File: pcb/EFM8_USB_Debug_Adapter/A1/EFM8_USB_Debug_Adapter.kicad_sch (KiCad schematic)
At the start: 27 parts, among them J100 EFM8 IDC Debug Header, J110 2137160001, J111 TTL-232R Header, J120 31230102, J130 EFM8 USB 8-Bit Debug Header, J131 Conn_01x02_Male, Q110 SI3443CDV-T1-GE3, Q111 DMMT5401, Q120 SI3443CDV-T1-GE3, Q121 DMMT5401, Q130 SI3443CDV-T1-GE3, Q131 DMMT5401

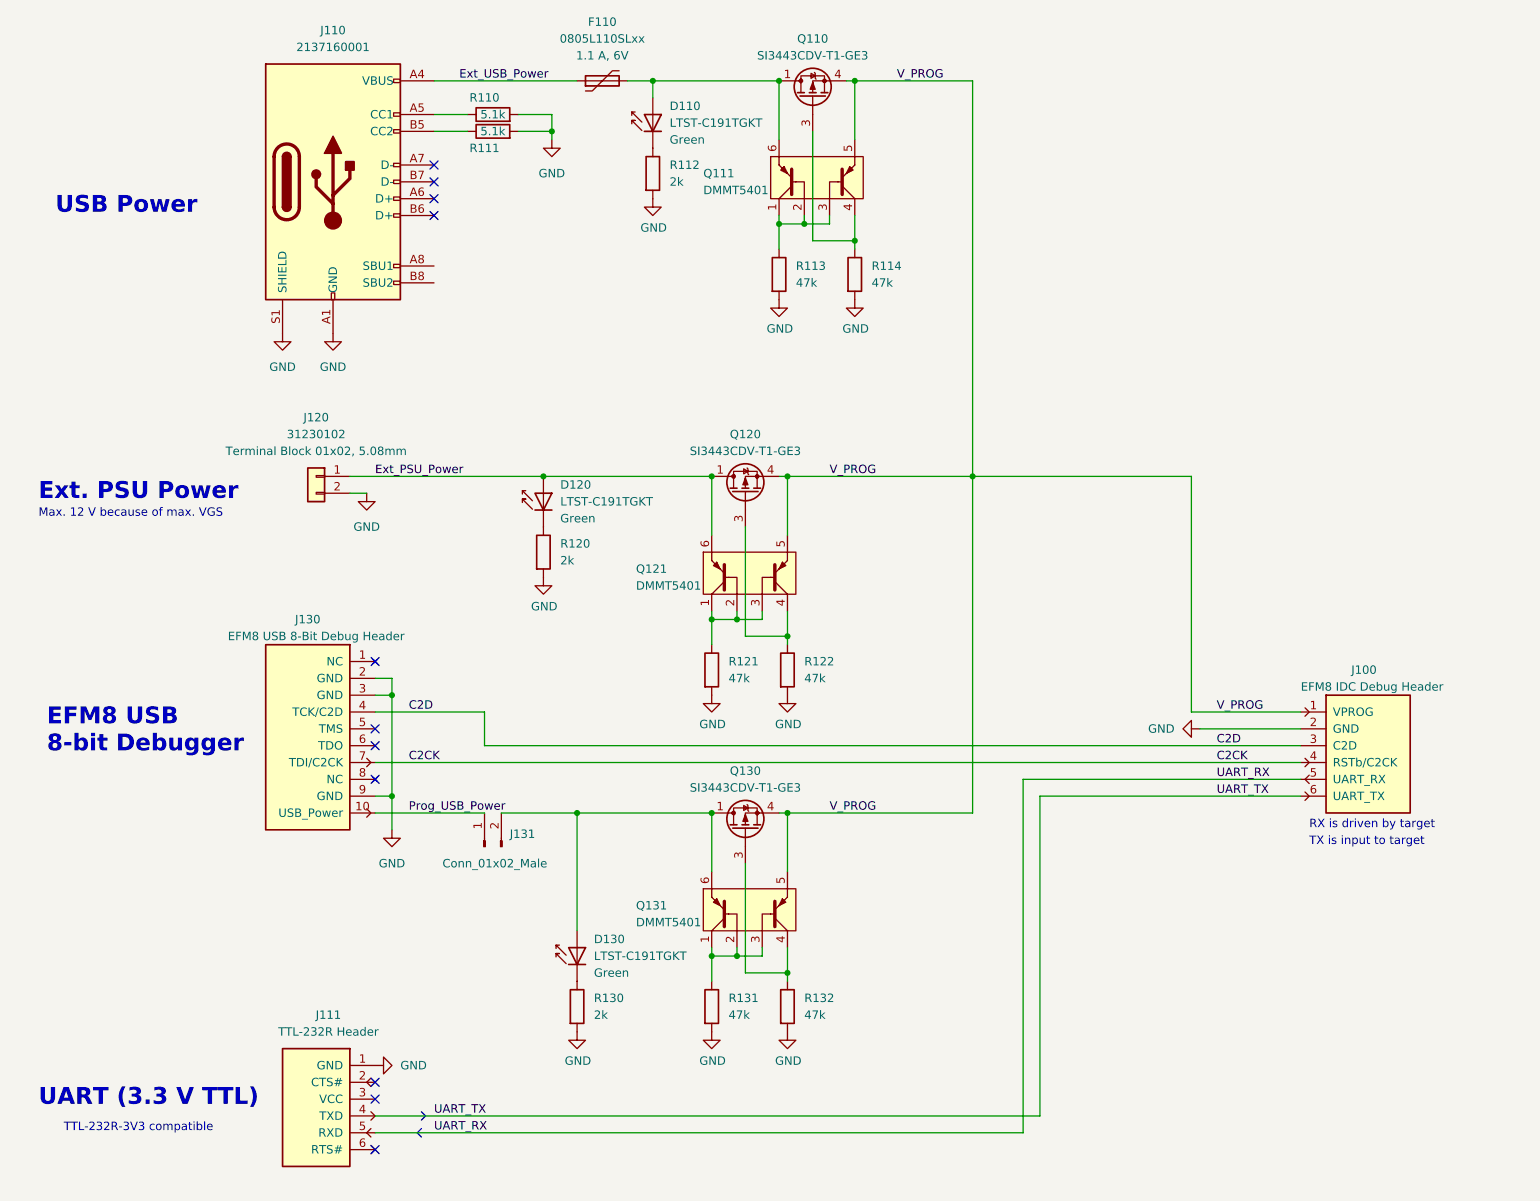
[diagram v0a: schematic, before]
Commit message: PCB bearbeitet, FreeCAD Projet angelegt
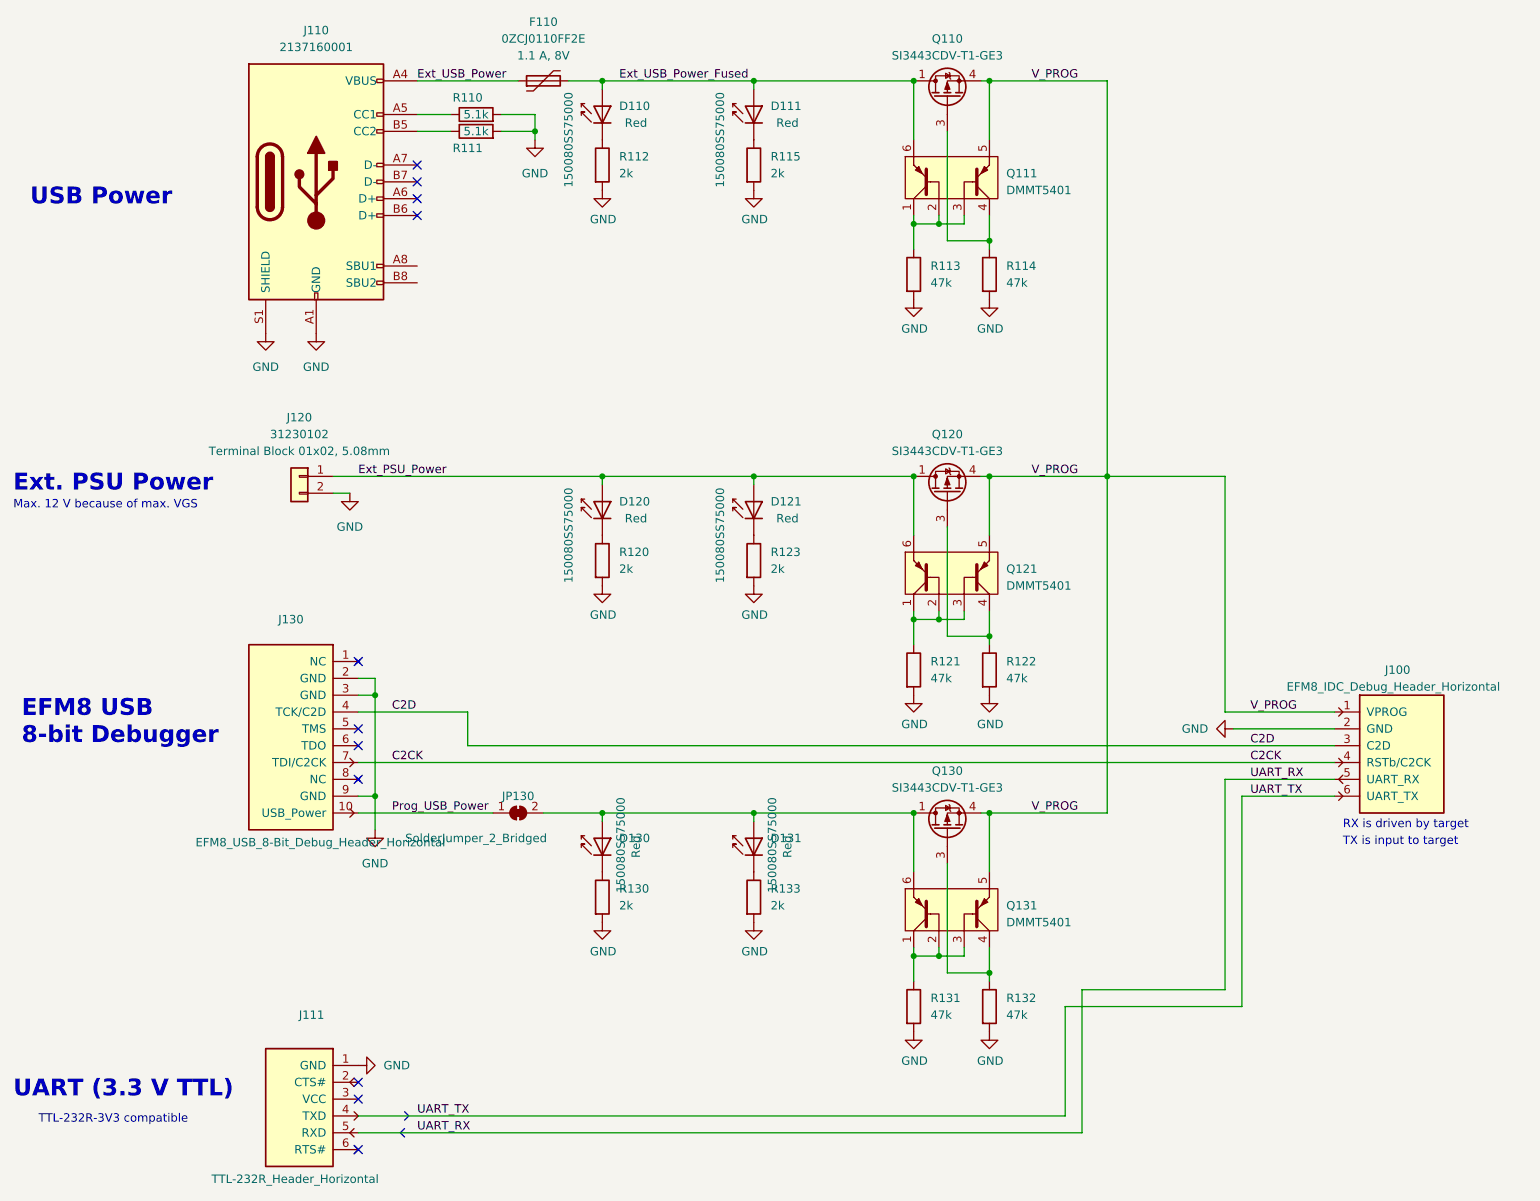
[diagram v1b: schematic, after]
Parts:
- removed F110: 0805L110SLxx, Fuse:Fuse_0805_2012Metric_Pad1.15x1.40mm_HandSolder, symbol Fuse_User:0805L110SLxx
- removed J131: Conn_01x02_Male, Connector_PinHeader_2.54mm:PinHeader_1x02_P2.54mm_Vertical, symbol Connector:Conn_01x02_Male
- added D111, D121, D131: 150080SS75000, LED_SMD:LED_0805_2012Metric_Pad1.15x1.40mm_HandSolder, symbol LED_User:150080SS75000
- added F110: 0ZCJ0110FF2E, Fuse:Fuse_1206_3216Metric_Pad1.42x1.75mm_HandSolder, symbol Fuse_User:0ZCJ0110FF2E
- added JP130: SolderJumper_2_Bridged, Jumper:SolderJumper-2_P1.3mm_Bridged_RoundedPad1.0x1.5mm, symbol Jumper:SolderJumper_2_Bridged
- added R115, R123, R133: 2k,0603, Resistor_SMD:R_0603_1608Metric_Pad0.98x0.95mm_HandSolder, symbol Resistor_User:2k,0603
- D110, D120, D130: value LTST-C191TGKT -> 150080SS75000; footprint LED_SMD:LED_0603_1608Metric_Pad1.05x0.95mm_HandSolder -> LED_SMD:LED_0805_2012Metric_Pad1.15x1.40mm_HandSolder; symbol LED_User:LTST-C191TGKT -> LED_User:150080SS75000; Info Green -> Red; Manufacturer Lite-On -> Wurth Elektronik; SPN 160-1888-1-ND -> 732-4985-1-ND
- J100: value EFM8 IDC Debug Header -> EFM8_IDC_Debug_Header_Horizontal; footprint Connector_User:IDC-Header_2x03_P2.54mm_Vertical_61200621621 -> Connector_User:IDC-Header_2x03_P2.54mm_Horizontal_61200621721; symbol Connector_Special_Purpose_User:EFM8 IDC Debug Header -> Connector_Special_Purpose_User:EFM8_IDC_Debug_Header_Horizontal; MPN 61200621621 -> 61200621721; SPN 732-5394-ND -> 732-5404-ND
- J111: value TTL-232R Header -> TTL-232R_Header_Horizontal; footprint Connector_PinHeader_2.54mm:PinHeader_1x06_P2.54mm_Vertical -> Connector_PinHeader_2.54mm:PinHeader_1x06_P2.54mm_Horizontal; symbol Connector_Special_Purpose_User:TTL-232R Header -> Connector_Special_Purpose_User:TTL-232R_Header_Horizontal; MPN 61300611121 -> 61300611021; Pretty Value 1 01x06 Header -> 01x06 Header, Vertical; SPN 732-5319-ND -> 732-5339-ND
- J130: value EFM8 USB 8-Bit Debug Header -> EFM8_USB_8-Bit_Debug_Header_Horizontal; footprint Connector_User:IDC-Header_2x05_P2.54mm_Vertical_61201021621 -> Connector_User:IDC-Header_2x05_P2.54mm_Horizontal_61201021721; symbol Connector_Special_Purpose_User:EFM8 USB 8-Bit Debug Header -> Connector_Special_Purpose_User:EFM8_USB_8-Bit_Debug_Header_Horizontal; MPN 61201021621 -> 61201021721; SPN 732-2094-ND -> 732-2098-ND
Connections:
- net Ext_PSU_Power: now also D121.2 (A)
- net Ext_USB_Power: now also F110.1
- net GND: now also R115.2, R123.2, R133.2
- net Prog_USB_Power: now also JP130.1 (A)
- net Ext_USB_Power_Fused: now reaches D110.2 (A), Q110.1 (D), Q110.2 (D), Q110.5 (D), Q110.6 (D), Q111.6 (E1)
- net Ext_USB_Power_Fused: now also D111.2 (A), F110.2
- net at D130.2 (A), Q130.1 (D), Q130.2 (D)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: now also D131.2 (A), JP130.2 (B)
- new net: D131.1 (K), R133.1
- new net: D121.1 (K), R123.1
- new net: D111.1 (K), R115.1
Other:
- moved on the sheet: D110, D120, D130, J100, J110, J111, J120, J130, Q110, Q111, Q120, Q121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
